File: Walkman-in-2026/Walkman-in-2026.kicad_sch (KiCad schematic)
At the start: 33 parts, among them J1 AudioJack3, J2 Micro_SD_Card, Q1 BSS138, Q2 BSS138, SW1 SW_Push, SW2 SW_Push, SW3 SW_Push, SW4 SW_SPST, SW5 SW_Push, SW6 SW_Push, U1 XIAO-ESP32-S3-DIP, U2 HS1602A-B, U3 PCM5102, U4 PCF8574P

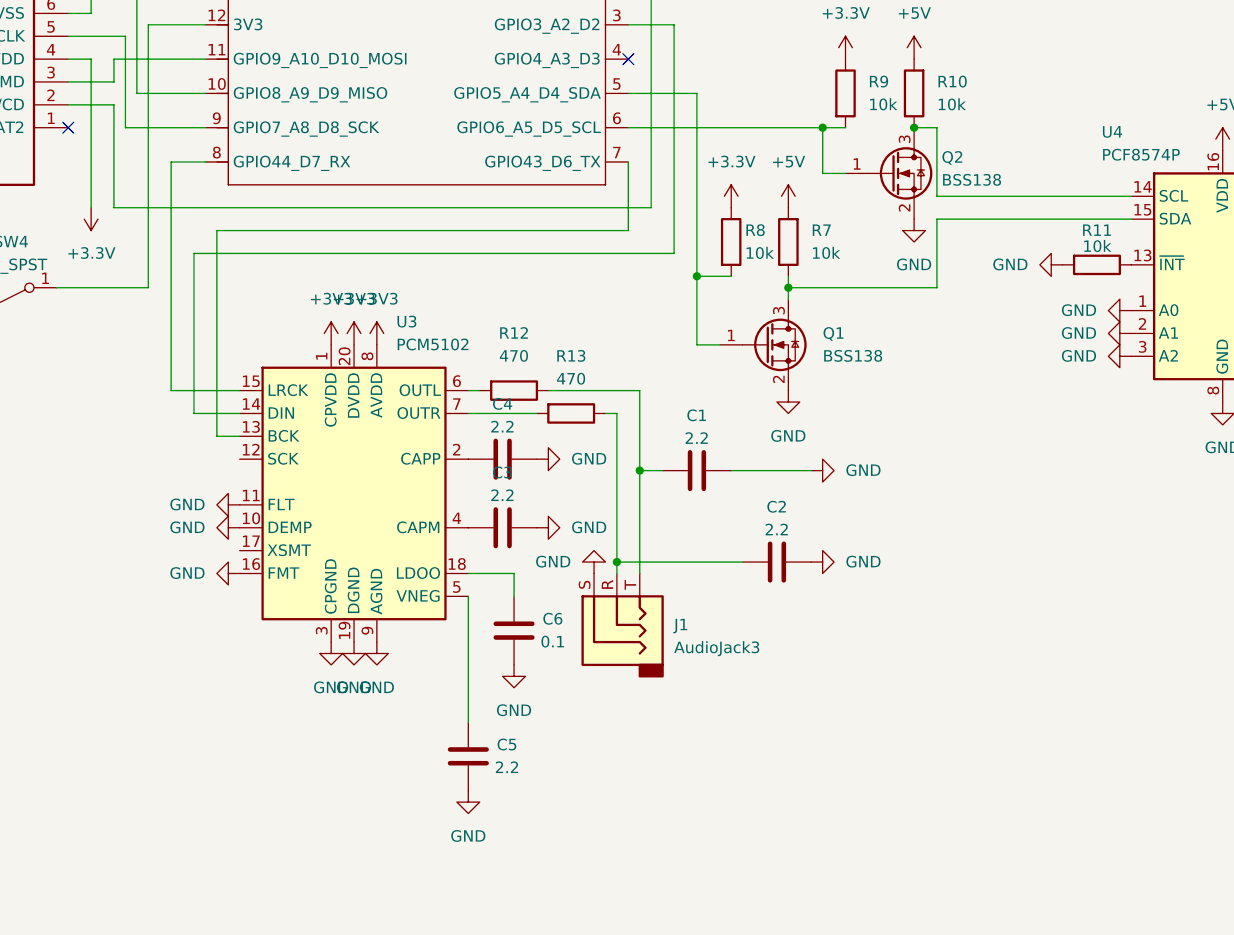
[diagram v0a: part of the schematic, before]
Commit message: jazz fest working
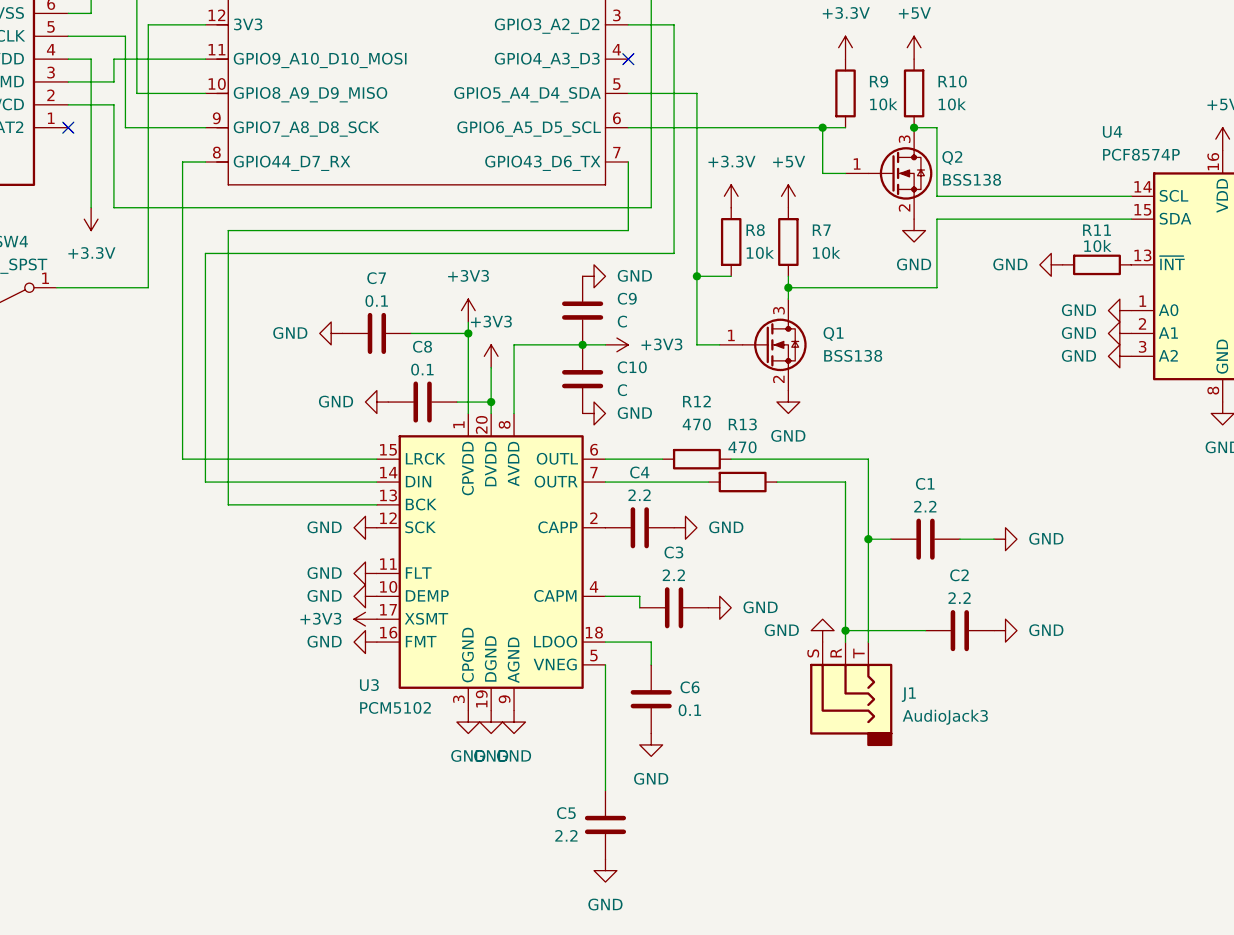
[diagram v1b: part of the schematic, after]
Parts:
- added C10, C9: C, symbol Device:C
- added C7, C8: 0.1, symbol Device:C
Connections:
- net +3V3: now also U3.17 (XSMT), C10.1, C7.2, C8.2, C9.2
- net GND: now also U3.12 (SCK), C10.2, C7.1, C8.1, C9.1
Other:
- moved on the sheet: C1, C2, C3, C4, C5, C6, J1, R12, R13, U3

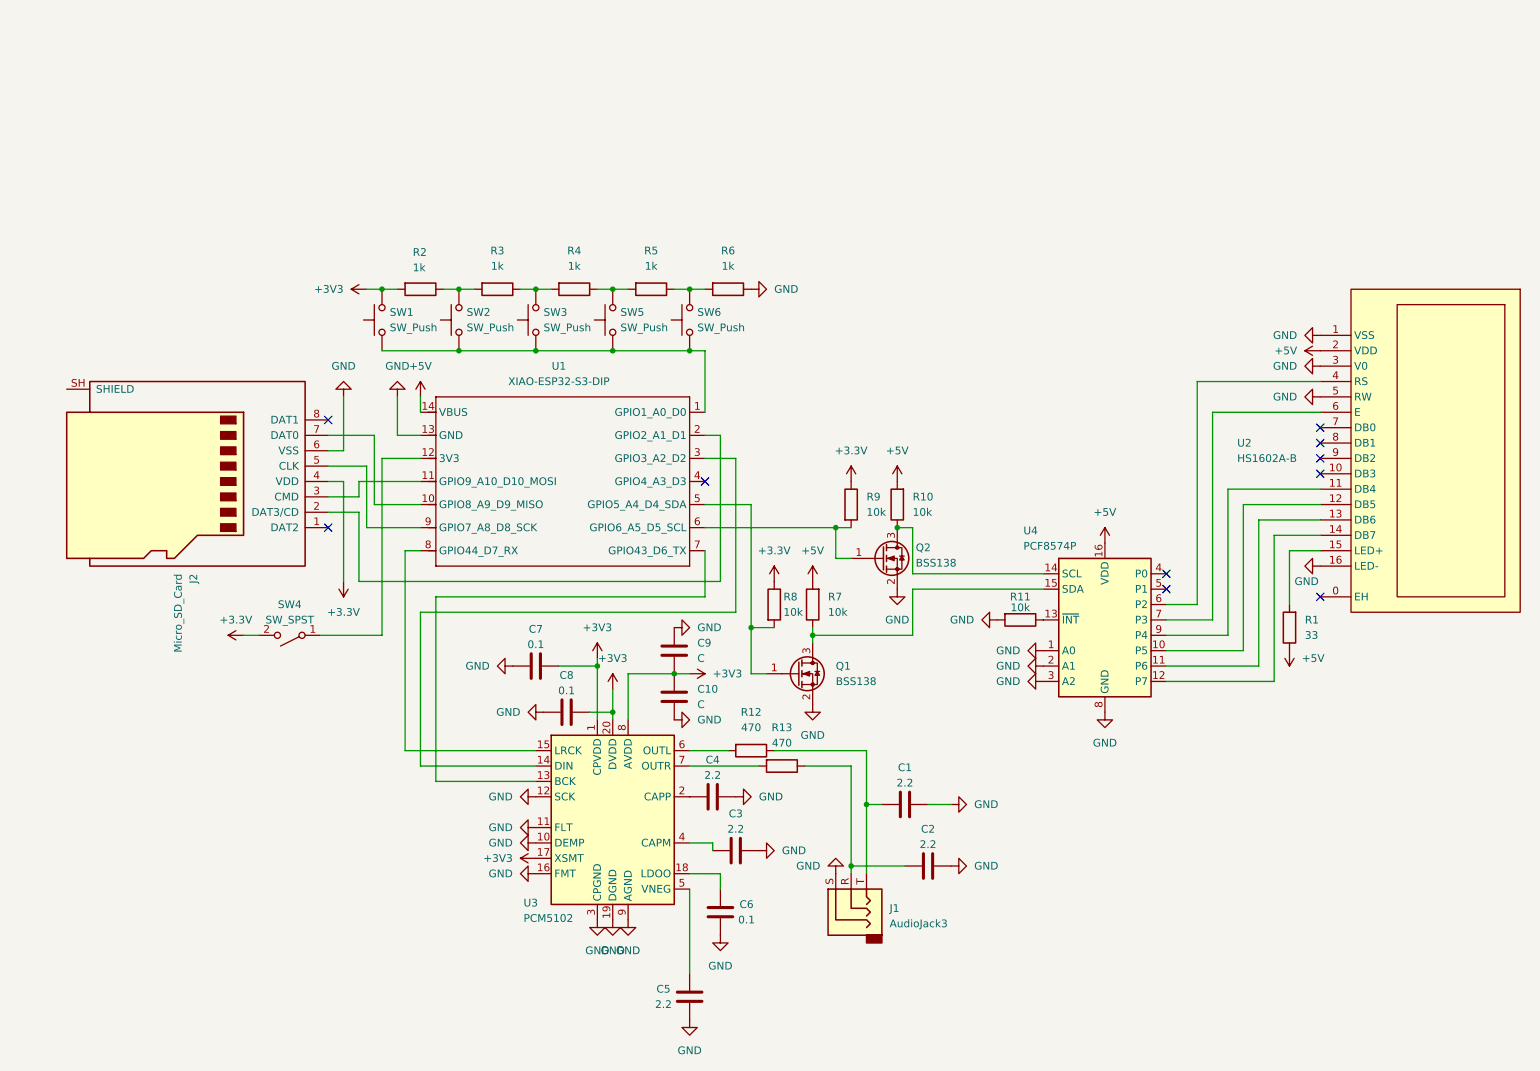
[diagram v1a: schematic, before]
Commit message: moving on to the pcb editor
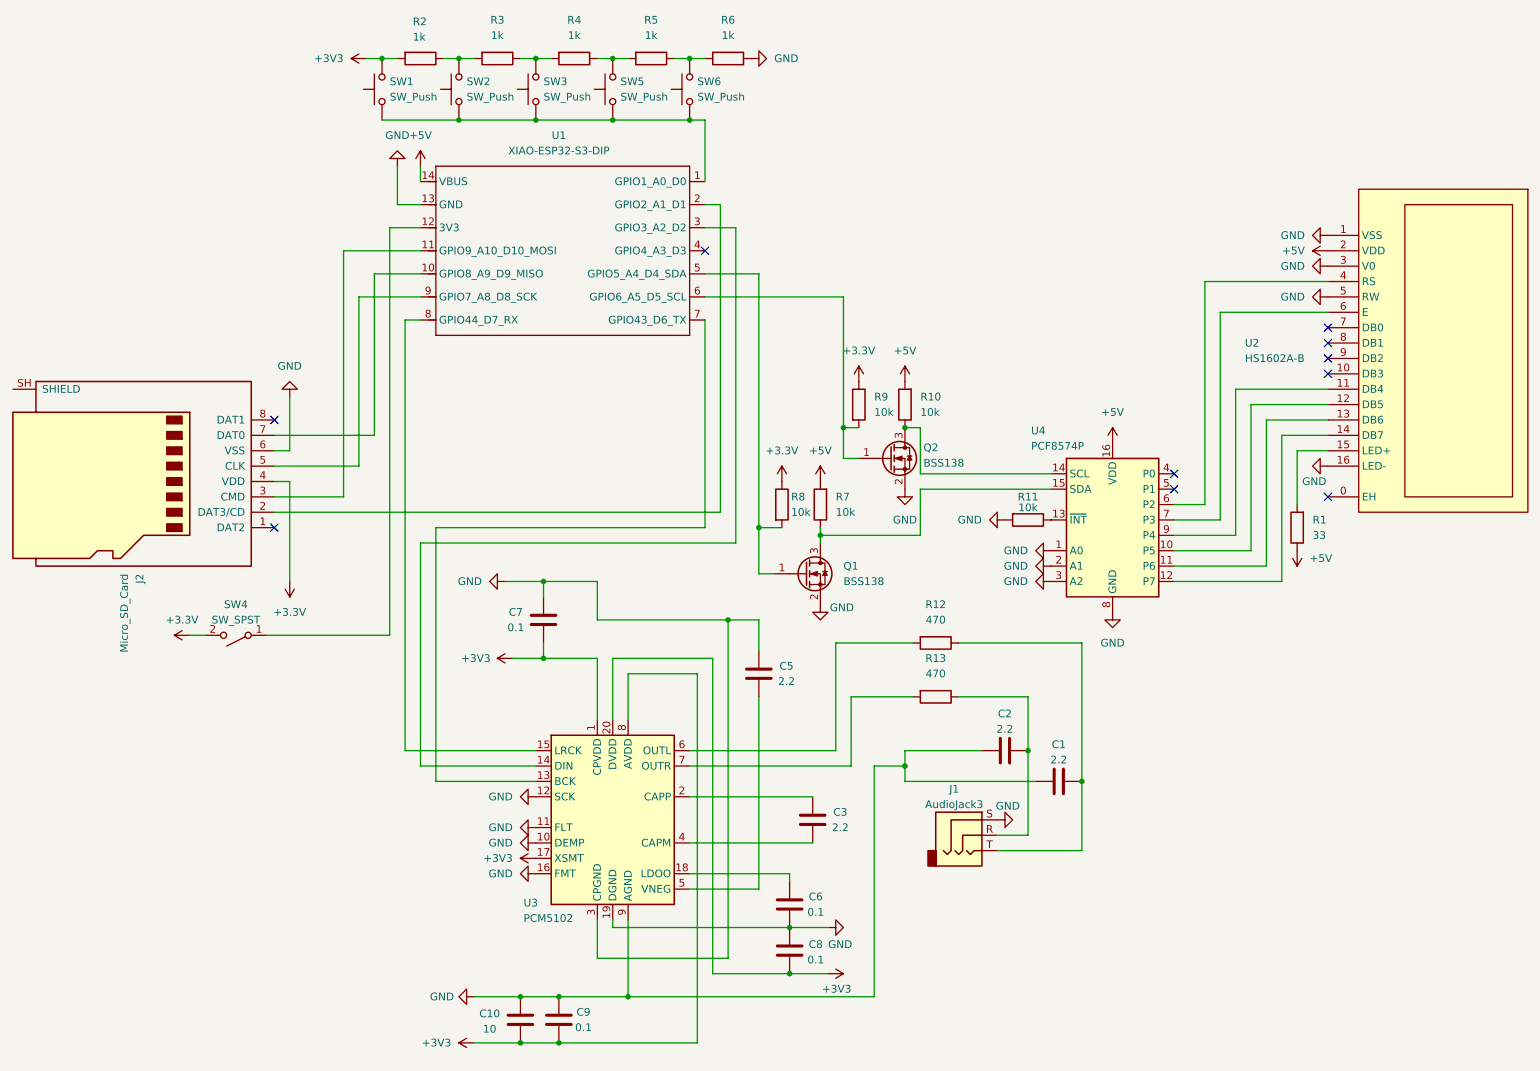
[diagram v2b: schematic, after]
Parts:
- removed C4: 2.2, symbol Device:C
- C1, C2, C6, C7, C8: footprint (none) -> Capacitor_THT:C_Disc_D3.0mm_W1.6mm_P2.50mm
- C10: value C -> 10; footprint (none) -> Capacitor_THT:C_Radial_D5.0mm_H5.0mm_P2.00mm
- C3, C5: footprint (none) -> Capacitor_THT:C_Radial_D5.0mm_H5.0mm_P2.00mm
- C9: value C -> 0.1; footprint (none) -> Capacitor_THT:C_Radial_D5.0mm_H5.0mm_P2.00mm
- J1: footprint (none) -> Connector_Audio:Jack_3.5mm_CUI_SJ1-3513N_Horizontal
- J2: footprint (none) -> Connector_Card:microSD_HC_Molex_47219-2001
- R1, R10, R11, R12, R13, R2, R3, R4, R5, R6, R7, R8, R9: footprint (none) -> Resistor_THT:R_Axial_DIN0207_L6.3mm_D2.5mm_P7.62mm_Horizontal
- SW1, SW2, SW3, SW5, SW6: footprint (none) -> Button_Switch_THT:SW_PUSH_6mm
- SW4: footprint (none) -> Button_Switch_THT:SW_SPST_Omron_B3F-315x_Angled
- U1: footprint Seeed_Studio_XIAO_Series:XIAO-ESP32-S3-DIP -> More_XIAO_Series_Footprints:XIAO-ESP32-S3-DIP
- U2: footprint easyeda2kicad:LCD1602 -> EasyEDALibrary:LCD1602
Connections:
- net GND: now also C1.1, C2.1; no longer C1.2, C2.2, C3.2
- net at J1.R, R13.1: now also C2.2; no longer C2.1
- net at U3.2 (CAPP): now also C3.1
- net at U3.4 (CAPM): now also C3.2; no longer C3.1
- net at J1.T, R12.1: now also C1.2; no longer C1.1
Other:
- moved on the sheet: C1, C2, C3, C5, C6, C7, C8, J1, J2, Q1, Q2, R1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
